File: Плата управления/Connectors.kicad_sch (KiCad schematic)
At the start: 15 parts, among them J1 A, J11 C, J12 C, J13 C, J14 C, J15 C, J16 Conn_02x05_Odd_Even, J2 B, J3 C, J4 Conn_01x10, J5 C, J6 Conn_01x02, J7 Conn_01x10, J8 Conn_01x02, J9 Conn_01x04

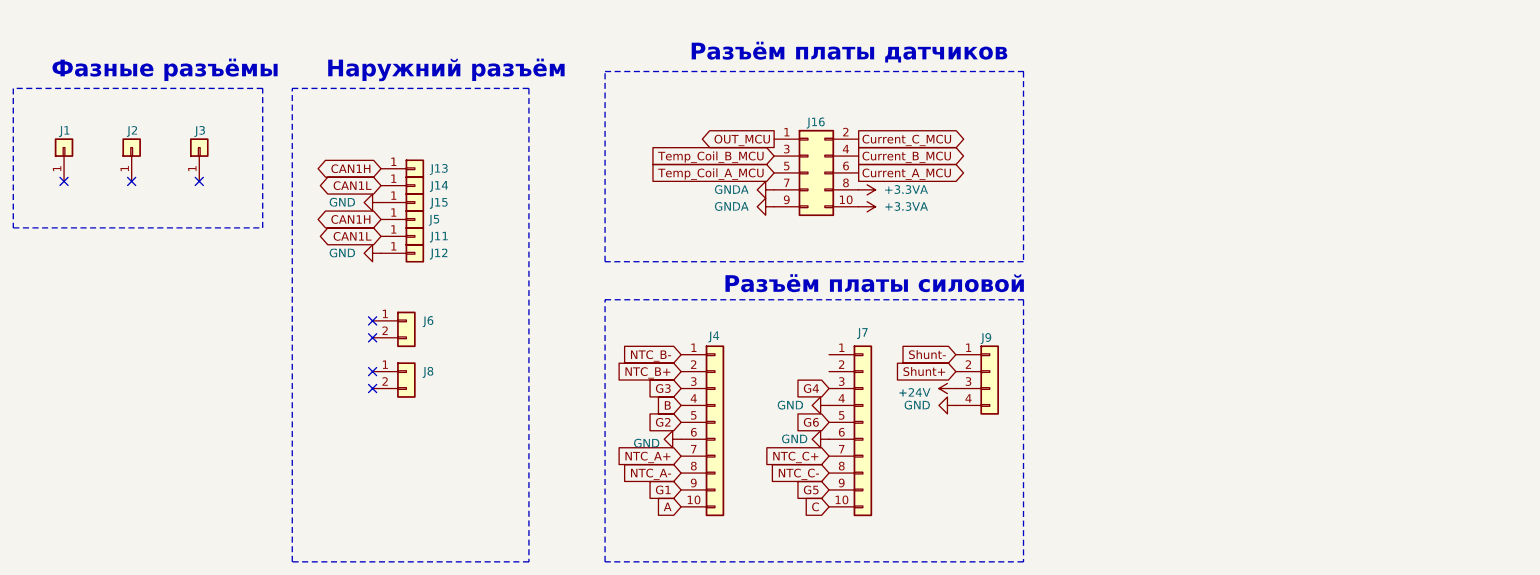
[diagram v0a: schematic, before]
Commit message: Изменения: добавил папку с отчетностью
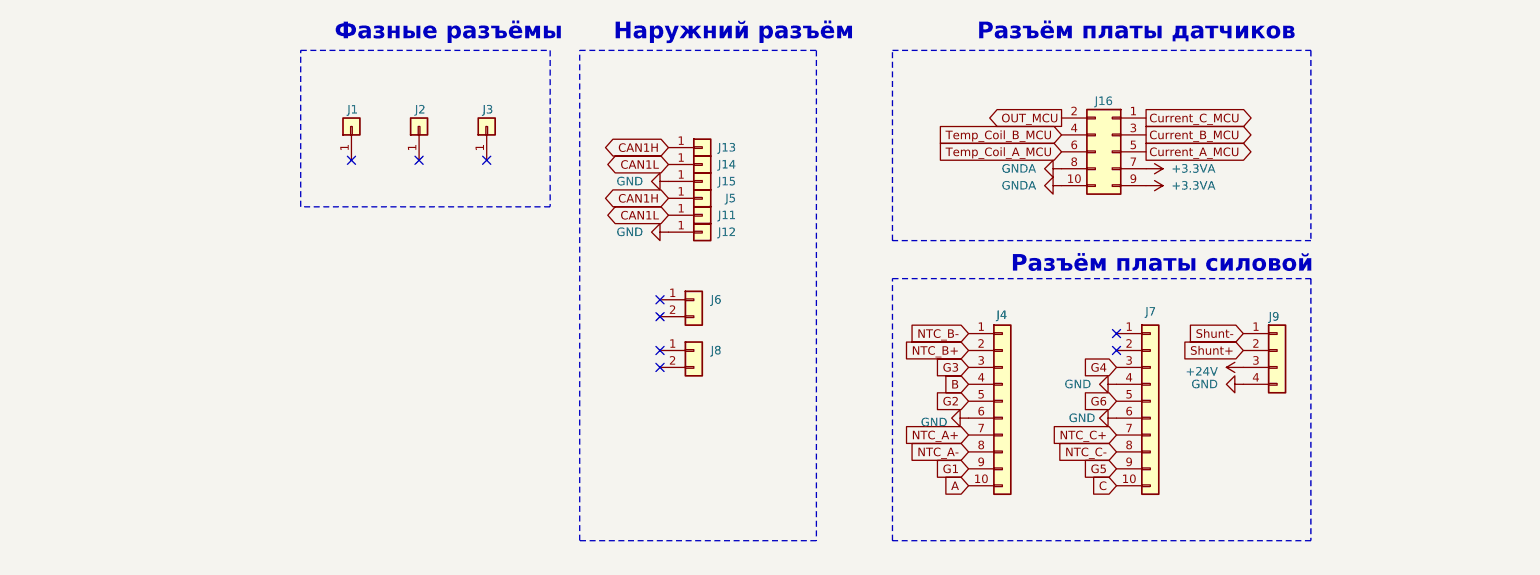
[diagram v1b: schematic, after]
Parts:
- J16: footprint Connector_PinSocket_1.27mm:PinSocket_2x05_P1.27mm_Vertical -> Connector_PinHeader_1.27mm:PinHeader_2x05_P1.27mm_Vertical
- J6, J8: footprint Connector_PinSocket_1.27mm:PinSocket_1x02_P1.27mm_Vertical -> Connector_PinHeader_1.27mm:PinHeader_1x02_P1.27mm_Vertical
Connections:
- net +3.3VA: now also J16.7 (Pin_7), J16.9 (Pin_9); no longer J16.10 (Pin_10), J16.8 (Pin_8)
- net Current_A_MCU: now also J16.5 (Pin_5); no longer J16.6 (Pin_6)
- net Current_B_MCU: now also J16.3 (Pin_3); no longer J16.4 (Pin_4)
- net Current_C_MCU: now also J16.1 (Pin_1); no longer J16.2 (Pin_2)
- net GNDA: now also J16.10 (Pin_10), J16.8 (Pin_8); no longer J16.7 (Pin_7), J16.9 (Pin_9)
- net OUT_MCU: now also J16.2 (Pin_2); no longer J16.1 (Pin_1)
- net Temp_Coil_A_MCU: now also J16.6 (Pin_6); no longer J16.5 (Pin_5)
- net Temp_Coil_B_MCU: now also J16.4 (Pin_4); no longer J16.3 (Pin_3)
- no-connect marks 7 -> 9
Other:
- moved on the sheet: J1, J11, J12, J13, J14, J15, J16, J2, J3, J4, J5, J6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
